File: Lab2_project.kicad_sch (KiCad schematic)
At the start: 45 parts, among them J1 PROG, J2 POWER IN, SW1 EC11B, SW2 RESET, SW3 BOOT, U1 STM32F407IGTx, U2 AMS1117-3.3, Y1 8 MHz

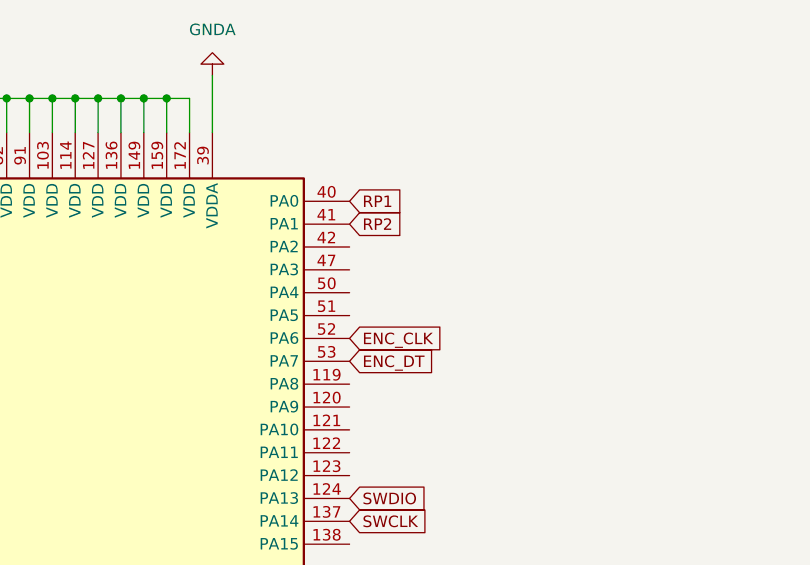
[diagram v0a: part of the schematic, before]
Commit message: fix: traced PCB
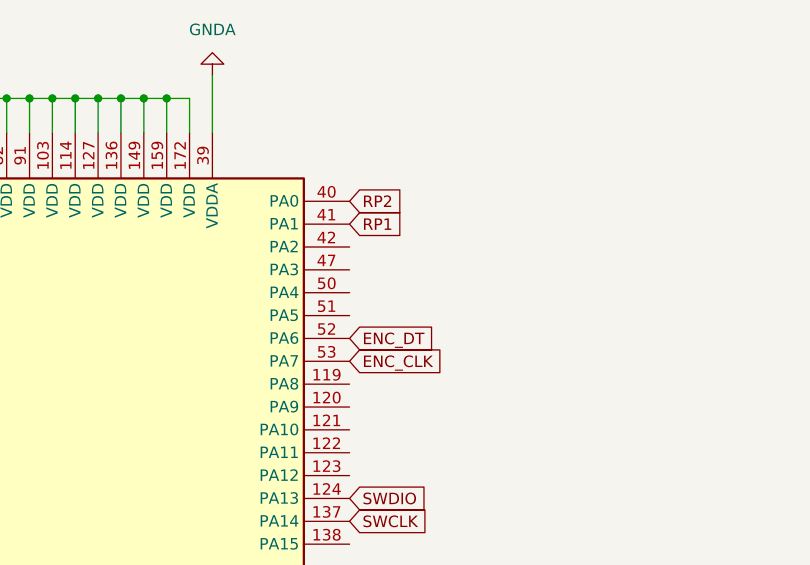
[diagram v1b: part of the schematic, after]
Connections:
- net ENC_CLK: now also U1.53 (PA7); no longer U1.52 (PA6)
- net ENC_DT: now also U1.52 (PA6); no longer U1.53 (PA7)
- net RP1: now also U1.41 (PA1); no longer U1.40 (PA0)
- net RP2: now also U1.40 (PA0); no longer U1.41 (PA1)
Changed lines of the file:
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@@
 	(global_label "RP2"
 		(shape input)
+		(at 158.75 43.18 0)
+		(fields_autoplaced yes)
+		(effects
+			(font
+				(size 1.27 1.27)
+			)
+			(justify left)
+		)
+		(property "Intersheetrefs" "${INTERSHEET_REFS}"
+			(at 165.4847 43.18 0)
+			(effects
+				(font
+					(size 1.27 1.27)
+				)
+				(justify left)
+				(hide yes)
+			)
+		)
+	)
+	(global_label "NRST"
+		(shape input)
+		(at 85.09 45.72 180)
+		(fields_autoplaced yes)
+		(effects
+			(font
+				(size 1.27 1.27)
+			)
+			(justify right)
+		)
+		(property "Intersheetrefs" "${INTERSHEET_REFS}"
+			(at 77.3272 45.72 0)
+			(effects
+				(font
+					(size 1.27 1.27)
+				)
+				(justify right)
+				(hide yes)
+			)
+		)
+	)
+	(global_label "SWCLK"
+		(shape input)
+		(at 158.75 78.74 0)
+		(fields_autoplaced yes)
+		(effects
+			(font
+				(size 1.27 1.27)
+			)
+			(justify left)
+		)
+		(property "Intersheetrefs" "${INTERSHEET_REFS}"
+			(at 167.9642 78.74 0)
+			(effects
+				(font
+					(size 1.27 1.27)
+				)
+				(justify left)
+				(hide yes)
+			)
+		)
+	)
+	(global_label "LED_B"
+		(shape input)
+		(at 158.75 210.82 0)
+		(fields_autoplaced yes)
+		(effects
+			(font
+				(size 1.27 1.27)
+			)
+			(justify left)
+		)
+		(property "Intersheetrefs" "${INTERSHEET_REFS}"
+			(at 167.4199 210.82 0)
+			(effects
+				(font
+					(size 1.27 1.27)
+				)
+				(justify left)
+				(hide yes)
+			)
+		)
+	)
+	(global_label "SWCLK"
+		(shape input)
+		(at 287.02 59.69 180)
+		(fields_autoplaced yes)
+		(effects
+			(font
+				(size 1.27 1.27)
+			)
+			(justify right)
+		)
+		(property "Intersheetrefs" "${INTERSHEET_REFS}"
+			(at 277.8058 59.69 0)
+			(effects
+				(font
+					(size 1.27 1.27)
+				)
+				(justify right)
+				(hide yes)
+			)
+		)
+	)
+	(global_label "ENC_DT"
+		(shape input)
+		(at 275.59 223.52 180)
+		(fields_autoplaced yes)
+		(effects
+			(font
+				(size 1.27 1.27)
+			)
+			(justify right)
+		)
+		(property "Intersheetrefs" "${INTERSHEET_REFS}"
+			(at 265.6501 223.52 0)
+			(effects
+				(font
+					(size 1.27 1.27)
+				)
+				(justify right)
+				(hide yes)
+			)
+		)
+	)
+	(global_label "LED_Y"
+		(shape input)
+		(at 236.22 189.23 180)
+		(fields_autoplaced yes)
+		(effects
+			(font
+				(size 1.27 1.27)
+			)
+			(justify right)
+		)
+		(property "Intersheetrefs" "${INTERSHEET_REFS}"
+			(at 227.7315 189.23 0)
+			(effects
+				(font
+					(size 1.27 1.27)
+				)
+				(justify right)
+				(hide yes)
+			)
+		)
+	)
+	(global_label "OSC_IN"
+		(shape input)
+		(at 85.09 96.52 180)
+		(fields_autoplaced yes)
+		(effects
+			(font
+				(size 1.27 1.27)
+			)
+			(justify right)
+		)
+		(property "Intersheetrefs" "${INTERSHEET_REFS}"
+			(at 75.3919 96.52 0)
+			(effects
+				(font
+					(size 1.27 1.27)
+				)
+				(justify right)
+				(hide yes)
+			)
+		)
+	)
+	(global_label "OSC_OUT"
+		(shape input)
+		(at 85.09 99.06 180)
+		(fields_autoplaced yes)
+		(effects
+			(font
+				(size 1.27 1.27)
+			)
+			(justify right)
+		)
+		(property "Intersheetrefs" "${INTERSHEET_REFS}"
+			(at 73.6986 99.06 0)
+			(effects
+				(font
+					(size 1.27 1.27)
+				)
+				(justify right)
+				(hide yes)
+			)
+		)
+	)
+	(global_label "RP1"
+		(shape input)
 		(at 158.75 45.72 0)
 		(fields_autoplaced yes)
@@
 		)
 	)
-	(global_label "NRST"
-		(shape input)
-		(at 85.09 45.72 180)
-		(fields_autoplaced yes)
-		(effects
-			(font
-				(size 1.27 1.27)
-			)
-			(justify right)
-		)
-		(property "Intersheetrefs" "${INTERSHEET_REFS}"
-			(at 77.3272 45.72 0)
-			(effects
-				(font
-					(size 1.27 1.27)
-				)
-				(justify right)
-				(hide yes)
-			)
-		)
-	)
-	(global_label "SWCLK"
-		(shape input)
-		(at 158.75 78.74 0)
-		(fields_autoplaced yes)
-		(effects
-			(font
-				(size 1.27 1.27)
-			)
-			(justify left)
-		)
-		(property "Intersheetrefs" "${INTERSHEET_REFS}"
-			(at 167.9642 78.74 0)
-			(effects
-				(font
-					(size 1.27 1.27)
-				)
-				(justify left)
-				(hide yes)
-			)
-		)
-	)
-	(global_label "LED_B"
-		(shape input)
-		(at 158.75 210.82 0)
-		(fields_autoplaced yes)
-		(effects
-			(font
-				(size 1.27 1.27)
-			)
-			(justify left)
-		)
-		(property "Intersheetrefs" "${INTERSHEET_REFS}"
-			(at 167.4199 210.82 0)
-			(effects
-				(font
-					(size 1.27 1.27)
-				)
-				(justify left)
-				(hide yes)
-			)
-		)
-	)
-	(global_label "SWCLK"
-		(shape input)
-		(at 287.02 59.69 180)
-		(fields_autoplaced yes)
-		(effects
-			(font
-				(size 1.27 1.27)
-			)
-			(justify right)
-		)
-		(property "Intersheetrefs" "${INTERSHEET_REFS}"
-			(at 277.8058 59.69 0)
-			(effects
-				(font
-					(size 1.27 1.27)
-				)
-				(justify right)
+	(global_label "OSC_OUT"
+		(shape input)
+		(at 248.92 66.04 0)
+		(fields_autoplaced yes)
+		(effects
+			(font
+				(size 1.27 1.27)
+			)
+			(justify left)
+		)
+		(property "Intersheetrefs" "${INTERSHEET_REFS}"
+			(at 260.3114 66.04 0)
+			(effects
+				(font
+					(size 1.27 1.27)
+				)
+				(justify left)
 				(hide yes)
 			)
@@
 	(global_label "ENC_DT"
 		(shape input)
-		(at 275.59 223.52 180)
-		(fields_autoplaced yes)
-		(effects
-			(font
-				(size 1.27 1.27)
-			)
-			(justify right)
-		)
-		(property "Intersheetrefs" "${INTERSHEET_REFS}"
-			(at 265.6501 223.52 0)
-			(effects
-				(font
-					(size 1.27 1.27)
-				)
-				(justify right)
-				(hide yes)
-			)
-		)
-	)
-	(global_label "LED_Y"
-		(shape input)
-		(at 236.22 189.23 180)
-		(fields_autoplaced yes)
-		(effects
-			(font
-				(size 1.27 1.27)
-			)
-			(justify right)
-		)
-		(property "Intersheetrefs" "${INTERSHEET_REFS}"
-			(at 227.7315 189.23 0)
-			(effects
-				(font
-					(size 1.27 1.27)
-				)
-				(justify right)
-				(hide yes)
-			)
-		)
-	)
-	(global_label "OSC_IN"
-		(shape input)
-		(at 85.09 96.52 180)
-		(fields_autoplaced yes)
-		(effects
-			(font
-				(size 1.27 1.27)
-			)
-			(justify right)
-		)
-		(property "Intersheetrefs" "${INTERSHEET_REFS}"
-			(at 75.3919 96.52 0)
-			(effects
-				(font
-					(size 1.27 1.27)
-				)
-				(justify right)
-				(hide yes)
-			)
-		)
-	)
-	(global_label "OSC_OUT"
-		(shape input)
-		(at 85.09 99.06 180)
-		(fields_autoplaced yes)
-		(effects
-			(font
-				(size 1.27 1.27)
-			)
-			(justify right)
-		)
-		(property "Intersheetrefs" "${INTERSHEET_REFS}"
-			(at 73.6986 99.06 0)
-			(effects
-				(font
-					(size 1.27 1.27)
-				)
-				(justify right)
-				(hide yes)
-			)
-		)
-	)
-	(global_label "RP1"
-		(shape input)
-		(at 158.75 43.18 0)
-		(fields_autoplaced yes)
-		(effects
-			(font
-				(size 1.27 1.27)
-			)
-			(justify left)
-		)
-		(property "Intersheetrefs" "${INTERSHEET_REFS}"
-			(at 165.4847 43.18 0)
-			(effects
-				(font
-					(size 1.27 1.27)
-				)
-				(justify left)
-				(hide yes)
-			)
-		)
-	)
-	(global_label "OSC_OUT"
-		(shape input)
-		(at 248.92 66.04 0)
-		(fields_autoplaced yes)
-		(effects
-			(font
-				(size 1.27 1.27)
-			)
-			(justify left)
-		)
-		(property "Intersheetrefs" "${INTERSHEET_REFS}"
-			(at 260.3114 66.04 0)
-			(effects
-				(font
-					(size 1.27 1.27)
-				)
-				(justify left)
-				(hide yes)
-			)
-		)
-	)
-	(global_label "ENC_DT"
+		(at 158.75 58.42 0)
+		(fields_autoplaced yes)
+		(effects
+			(font
+				(size 1.27 1.27)
+			)
+			(justify left)
+		)
+		(property "Intersheetrefs" "${INTERSHEET_REFS}"
+			(at 168.6899 58.42 0)
+			(effects
+				(font
+					(size 1.27 1.27)
+				)
+				(justify left)
+				(hide yes)
+			)
+		)
+	)
+	(global_label "ENC_CLK"
 		(shape input)
 		(at 158.75 60.96 0)
@@
 		)
 		(property "Intersheetrefs" "${INTERSHEET_REFS}"
-			(at 168.6899 60.96 0)
-			(effects
-				(font
-					(size 1.27 1.27)
-				)
-				(justify left)
-				(hide yes)
-			)
-		)
-	)
-	(global_label "ENC_CLK"
-		(shape input)
-		(at 158.75 58.42 0)
-		(fields_autoplaced yes)
-		(effects
-			(font
-				(size 1.27 1.27)
-			)
-			(justify left)
-		)
-		(property "Intersheetrefs" "${INTERSHEET_REFS}"
-			(at 170.0204 58.42 0)
-			(effects
-				(font
+			(at 170.0204 60.96 0)
+			(effects
+				(font
